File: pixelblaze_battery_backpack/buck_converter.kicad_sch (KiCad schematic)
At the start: 15 parts, among them U5 TPS54560BDDA

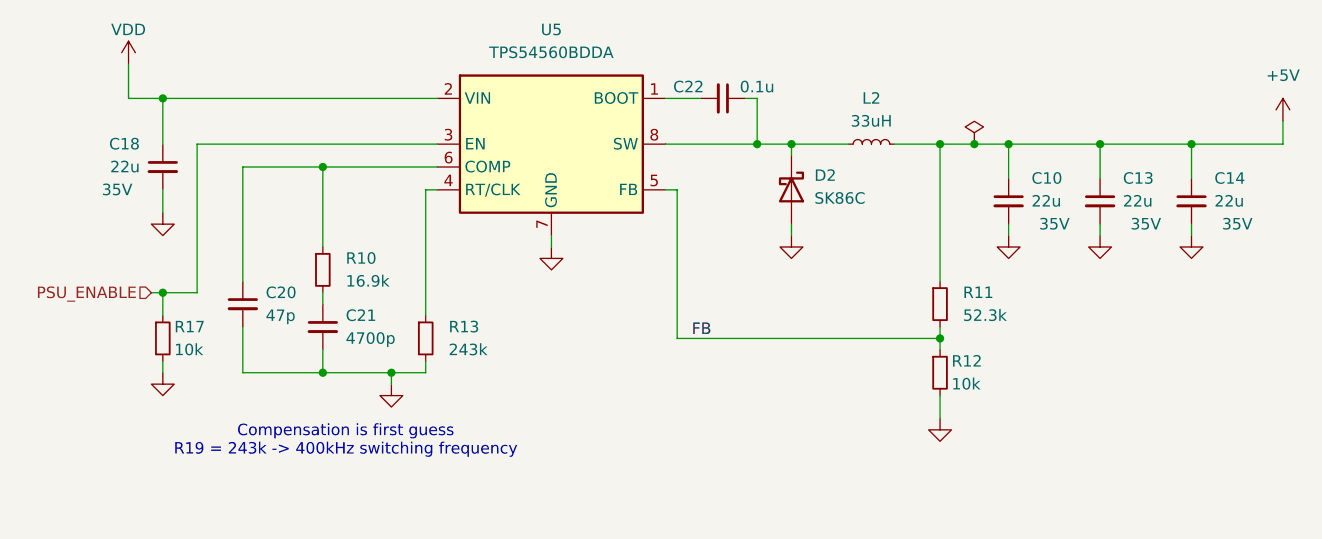
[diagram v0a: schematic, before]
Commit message: Checkpoint, changing computers
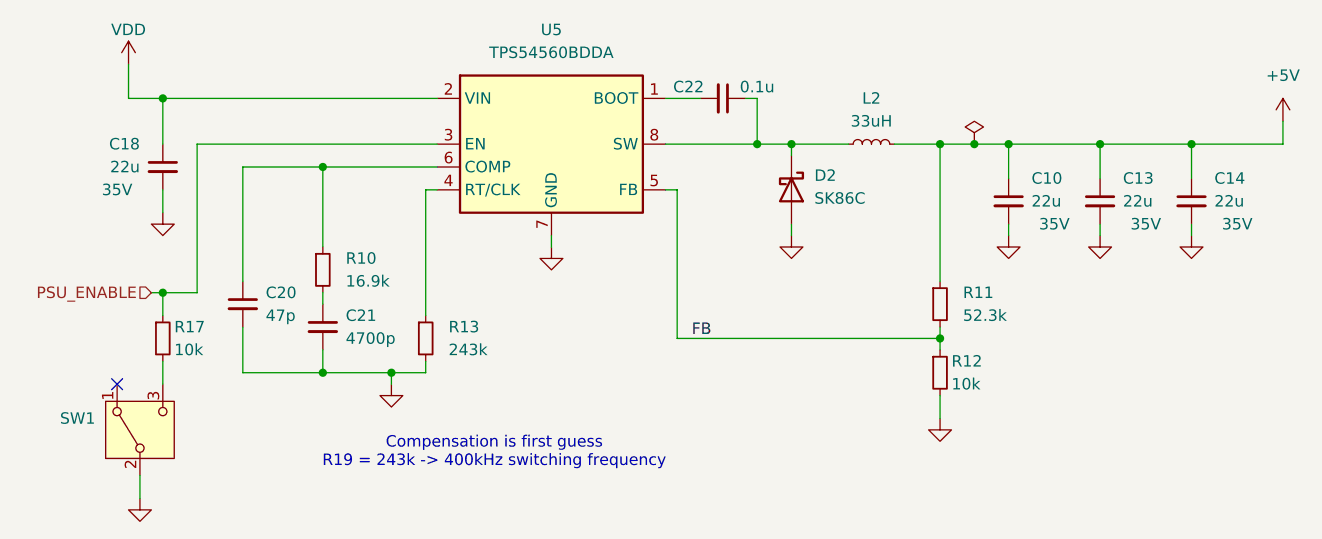
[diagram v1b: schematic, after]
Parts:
- added SW1: SW_SPDT, Button_Switch_SMD:SW_SPDT_Shouhan_MSK12C02, symbol Switch:SW_SPDT
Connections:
- net GND: now also SW1.2 (B); no longer R17.2
- new net: R17.2, SW1.3 (C)
- no-connect marks 0 -> 1
